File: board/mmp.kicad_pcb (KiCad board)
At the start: 2 copper layers, 50 x 32 mm, 65 parts, among them IC1 STM32F103C, IC2 SI8662, IC3 SI8662, IC4 MCP1700-33, IC5 MCP1700-33, IC6 TXS0108, IC7 1117-SOT223, J1 SWD, P1 USB_B, P2 CONN_01X04, P3 TC2030-CTX, Q1 2n2007, Q2 NTR4101, SW1 SW_PUSH, SW2 SP3T, SW3 SW_PUSH, U2 ROE-0505S, Y1 Crystal_Small

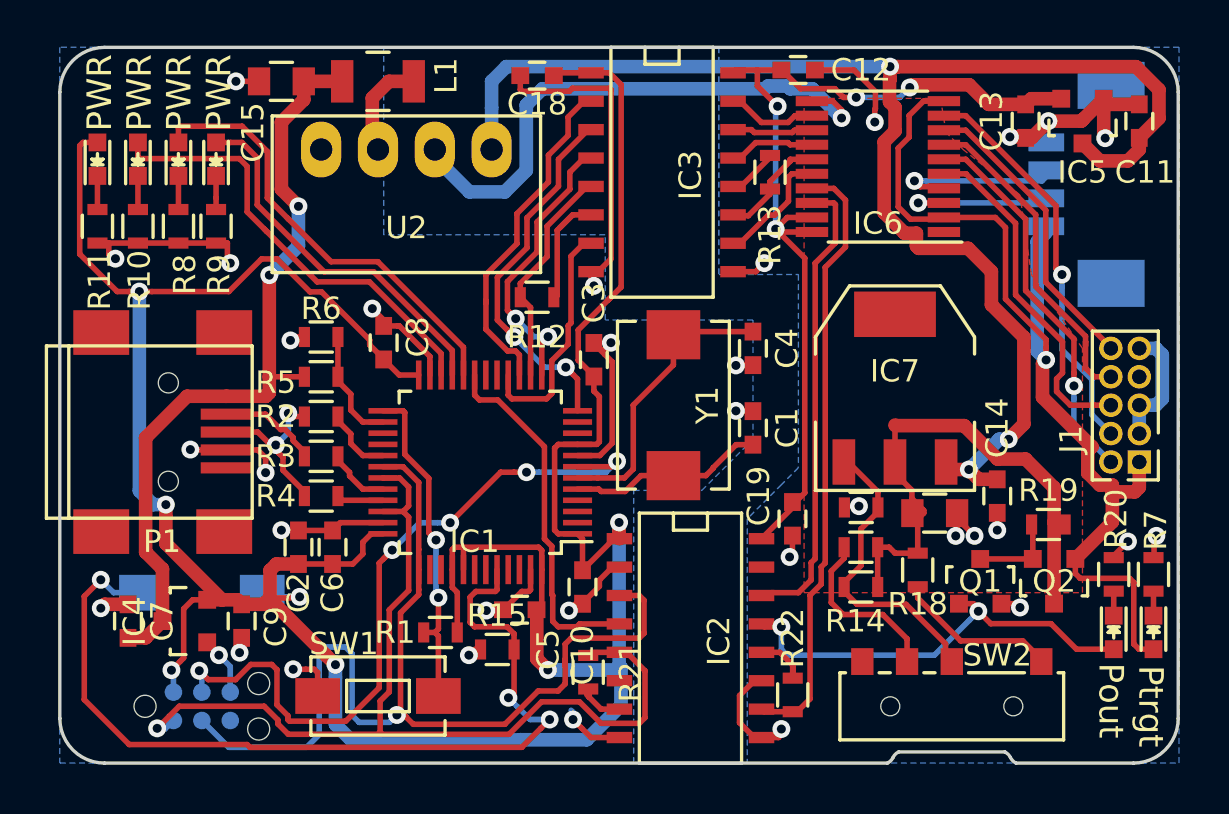
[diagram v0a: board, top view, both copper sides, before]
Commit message: finishing off
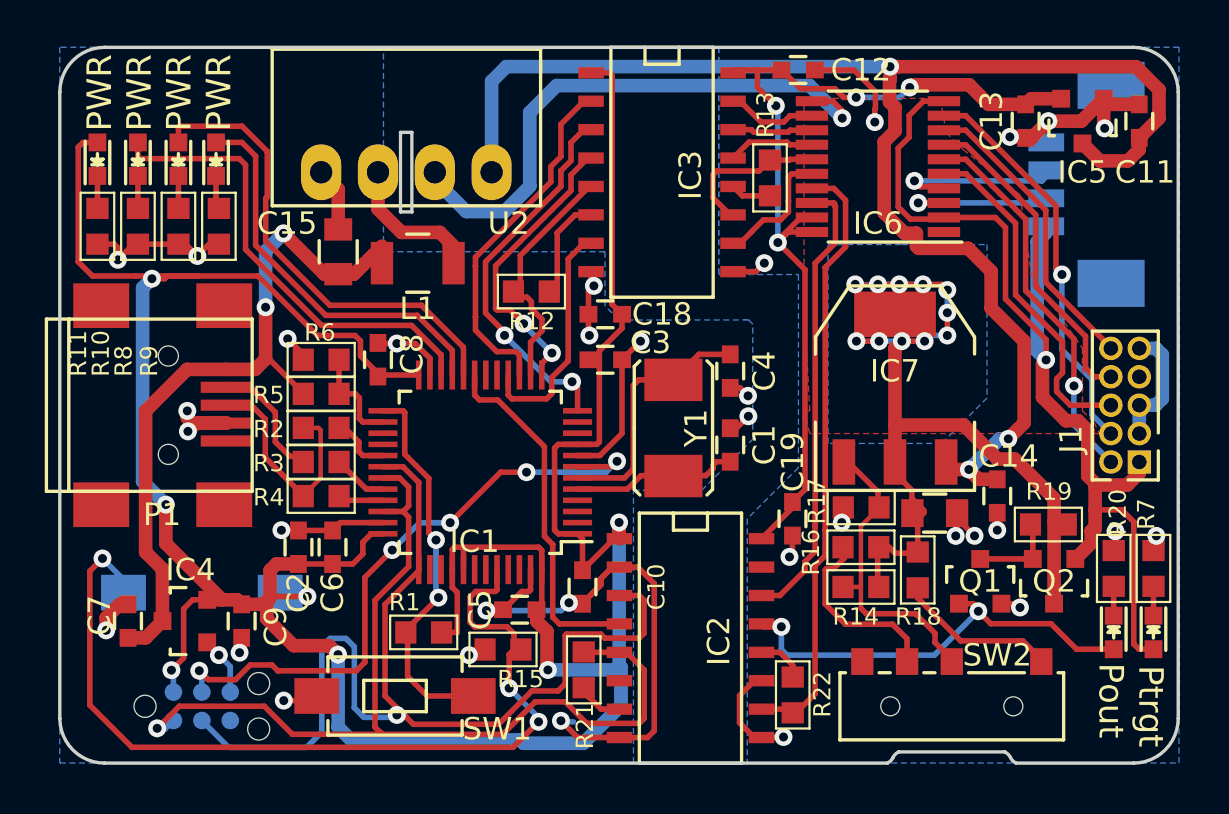
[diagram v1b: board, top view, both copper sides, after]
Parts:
- R1, R10, R11, R12, R13, R14, R15, R16, R17, R18, R19, R2, R20, R21, R22, R3, R4, R5, R6, R7, R8, R9: footprint Resistors_SMD:R_0603 -> passives-7351:C0603-N
- SW1, SW3: footprint Buttons_Switches_SMD:SW_SPST_EVQPE1 -> tactile_SPST:SW_SPST_EVQPE1
- Y1: footprint Crystals:Crystal_FOX-FE_SMD -> ABM7:ABM7
- moved C18 11.1 mm to (202.4, 70.9)
- moved L1 8.32 mm to (194.0, 68.6)
- moved C15 8.03 mm to (190.4, 68.1), turned to 90 degrees
- moved C4 1.44 mm to (208.0, 73.5)
- moved C1 1.27 mm to (208.0, 76.8)
- moved P1 1.20 mm to (182.0, 75.0)
- moved U2 1.02 mm to (193.5, 64.6)
- moved R6 1.02 mm to (189.7, 73.0)
- moved Y1 1.02 mm to (205.4, 76.0)
- moved C8 0.80 mm to (192.2, 73.0)
- moved R5 0.76 mm to (189.7, 74.5)
- moved SW1 0.76 mm to (193.0, 88.0)
- moved R1 0.75 mm to (194.3, 85.2)
- moved R2 0.51 mm to (189.7, 76.0)
- moved C3 0.51 mm to (202.4, 73.0), turned to 0 degrees
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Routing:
- net /REGOUT: track 24.0 -> 42.9 mm, vias 0 -> 11
- net GND: track 62.6 -> 68.5 mm
- net /H_RST: track 32.7 -> 28.2 mm
- net /Vbus: track 35.2 -> 31.9 mm
- net Net-(IC1-Pad25): track 14.9 -> 17.6 mm
- net Net-(P1-Pad3): track 7.99 -> 10.6 mm, vias 2 -> 0
- net Net-(IC3-Pad11): track 4.97 -> 7.00 mm
- net Net-(C4-Pad1): track 13.0 -> 11.3 mm
- net +3V3: track 137.9 -> 139.5 mm
- net Net-(C1-Pad1): track 8.77 -> 7.42 mm
- net Net-(C16-Pad2): track 4.57 -> 5.71 mm
- net /LED0: track 20.1 -> 21.2 mm
- net /LED1: track 16.7 -> 17.8 mm
- net Net-(P1-Pad2): track 4.46 -> 5.54 mm
- net Net-(IC3-Pad6): track 5.71 -> 4.83 mm
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- added copper zone on B.Cu, net /REGOUT
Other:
- outline, holes or cut-outs redrawn
